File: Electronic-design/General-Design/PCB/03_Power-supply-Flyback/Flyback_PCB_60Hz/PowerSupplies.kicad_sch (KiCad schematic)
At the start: 26 parts, among them IC1 TPS54302DDCR, IC2 L7812CV, IC3 L7912CV, J2 -12V, J3 +12V, J4 +5V, T1 3FS-324

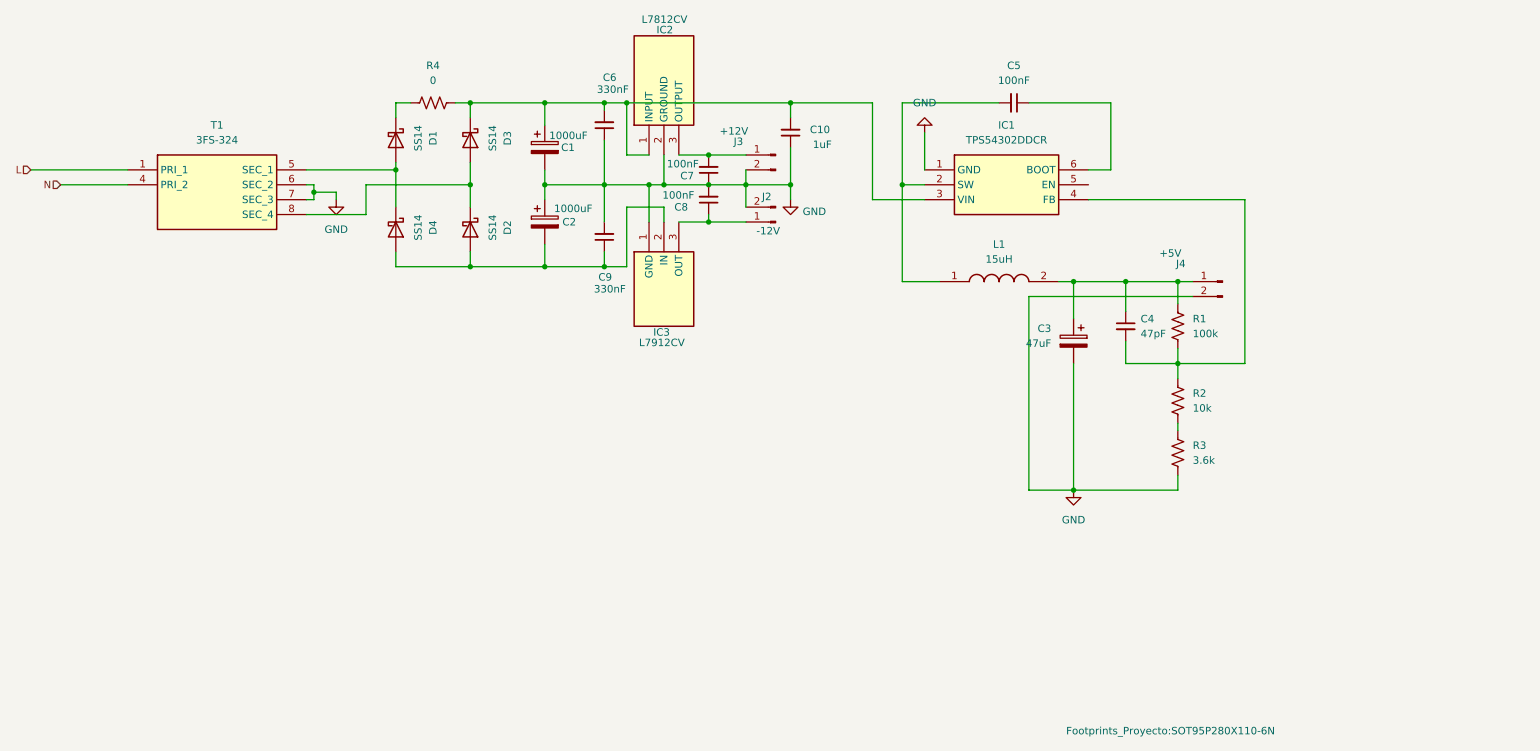
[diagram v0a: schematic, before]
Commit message: PSIM-FLYBACK-FINAL
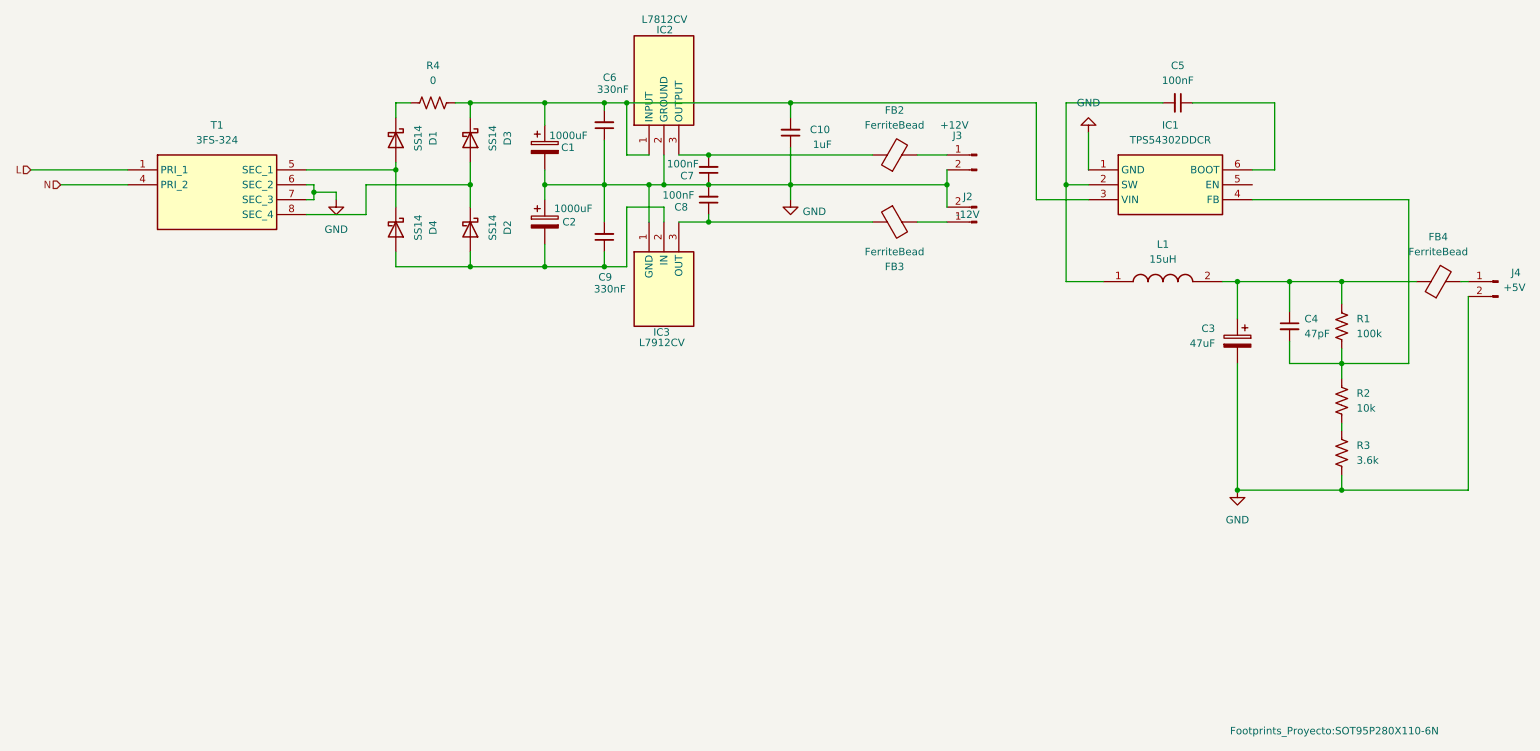
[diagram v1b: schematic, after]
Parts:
- added FB2, FB3, FB4: FerriteBead, Flyback:BEADC1608X95N, symbol Device:FerriteBead
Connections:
- net at C7.2, IC2.3 (OUTPUT): now also FB2.1; no longer J3.1 (Pin_1)
- net at C8.1, IC3.3 (OUT): now also FB3.1; no longer J2.1 (Pin_1)
- net at C3.1, C4.1, L1.2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: now also FB4.1; no longer J4.1 (Pin_1)
- new net: FB2.2, J3.1 (Pin_1)
- new net: FB3.2, J2.1 (Pin_1)
- new net: FB4.2, J4.1 (Pin_1)
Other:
- moved on the sheet: C3, C4, C5, IC1, J2, J3, J4, L1, R1, R2, R3
